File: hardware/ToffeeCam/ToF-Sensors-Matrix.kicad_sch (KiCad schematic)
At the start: 17 parts, among them Q601 AO3401A

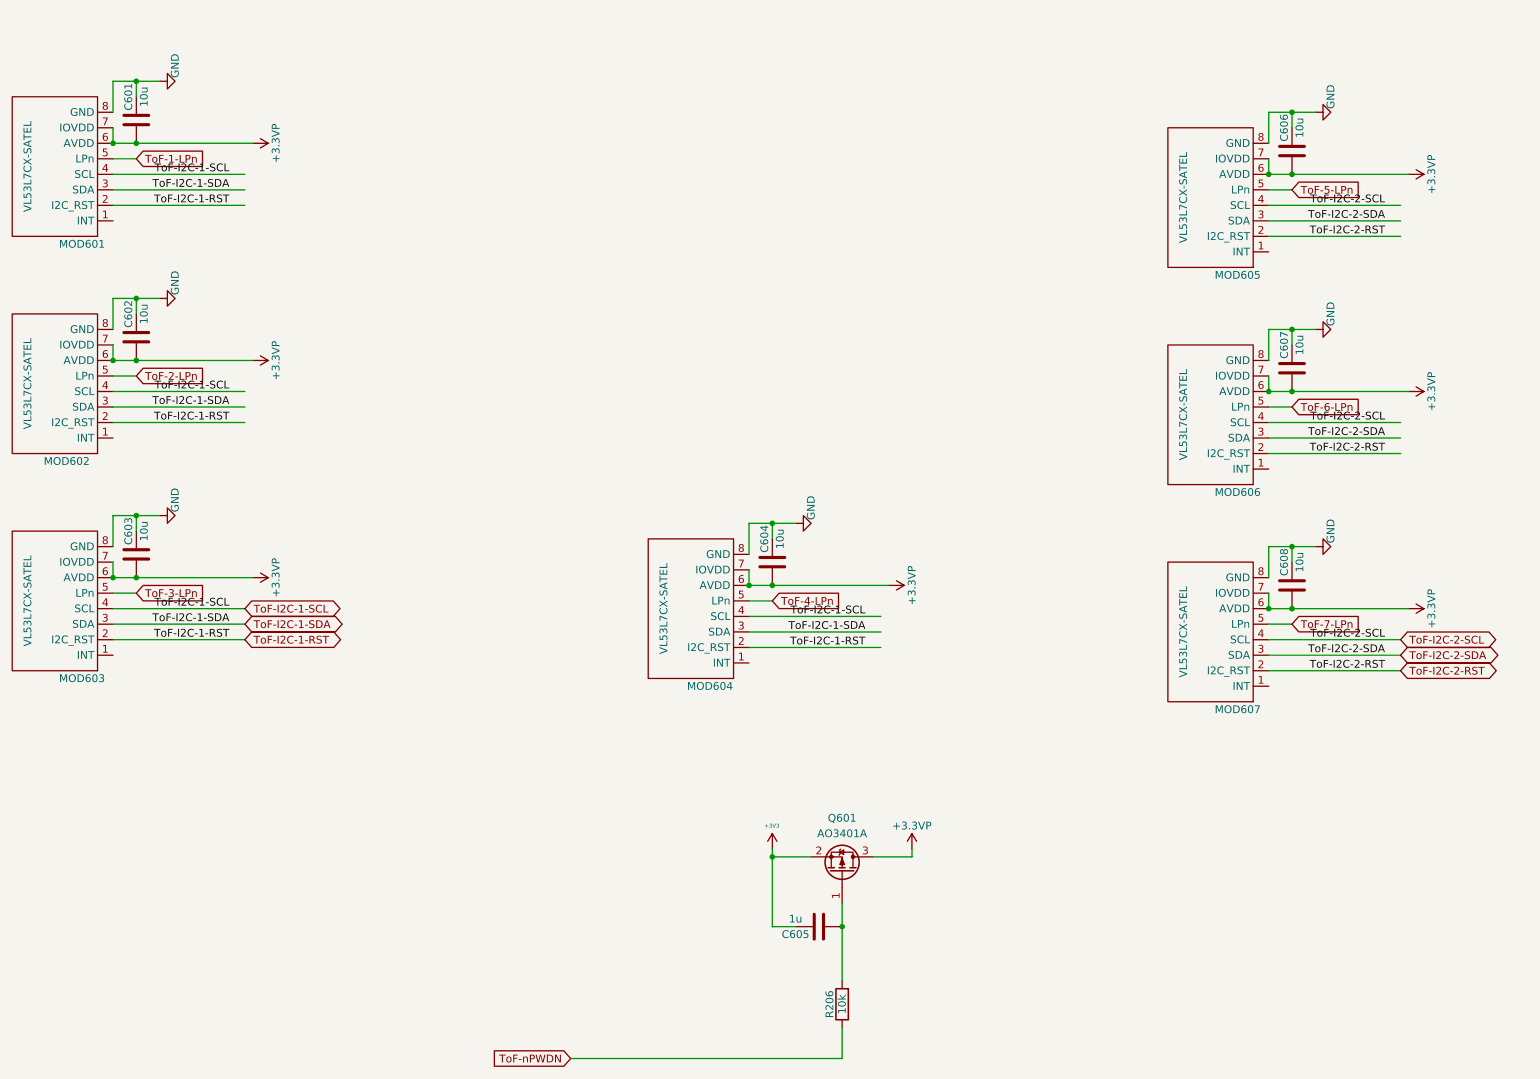
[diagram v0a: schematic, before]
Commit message: Clean schematics
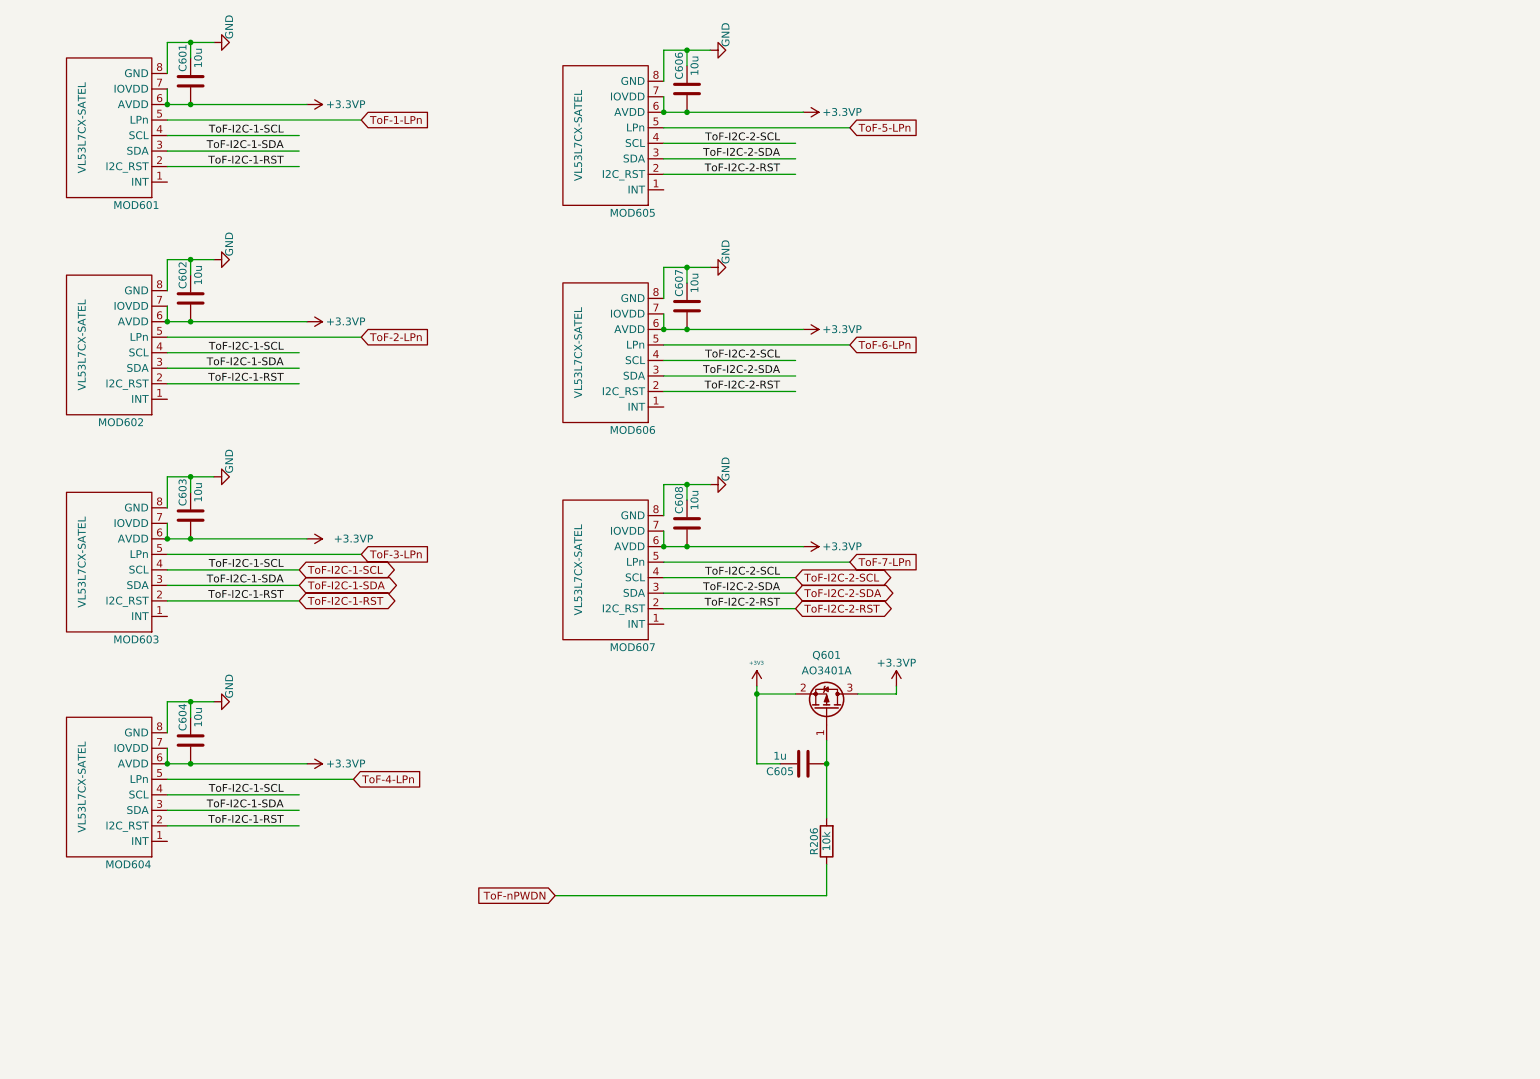
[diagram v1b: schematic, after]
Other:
- moved on the sheet: C601, C602, C603, C604, C605, C606, C607, C608, MOD601, MOD602, MOD603, MOD604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
